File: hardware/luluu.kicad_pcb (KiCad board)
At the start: 4 copper layers, 75 x 30 mm, 55 parts, among them J1 BATT_CON, J2 RPi SWD, J3 STEMMA_{QT} I_{2}C, J4 Micro_SD_Card, J6 USB_C_Receptacle_USB2.0, J7 DISP_LCD_ST7789, Q1 AO3401A, Q2 BSS138, SW1 SW_USBBOOT, SW2 SW_RESET, SW3 SW_POWER, U1 W25Q128JVSS, U2 RT9080-33GJ5, U3 RP2040, U4 TP4054-42, Y1 X322512MSB4SI

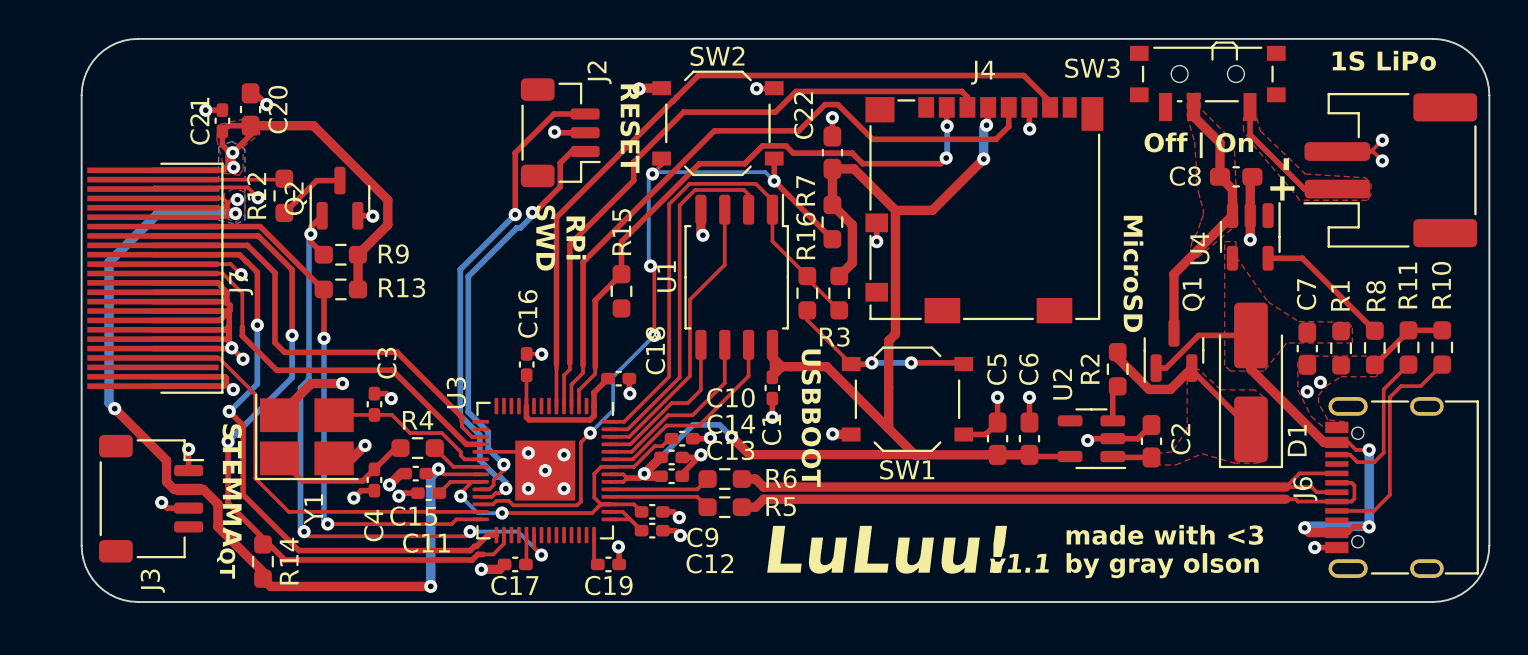
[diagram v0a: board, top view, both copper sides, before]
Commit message: pcb rev 2.0 progress
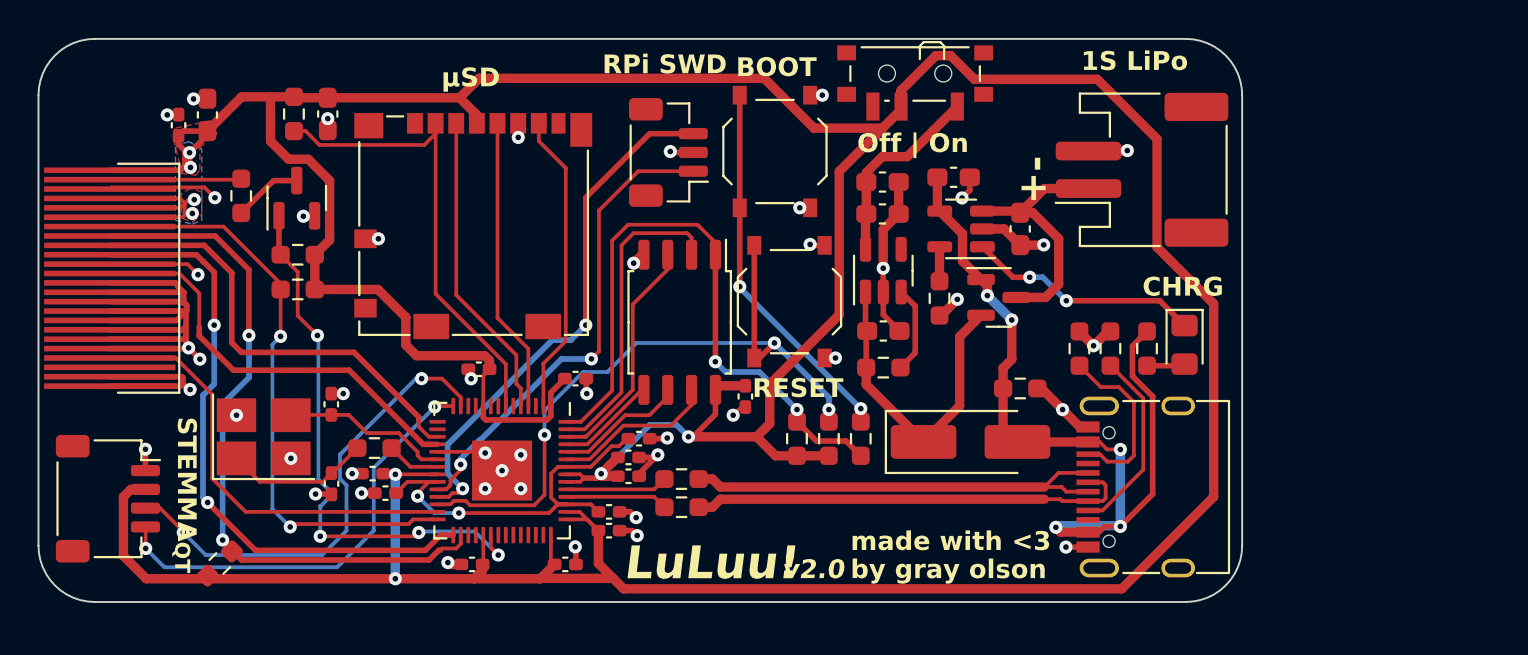
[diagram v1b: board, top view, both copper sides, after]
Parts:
- added D2: CHRG, LED_SMD:LED_0805_2012Metric_Pad1.15x1.40mm_HandSolder, F.Cu at (171.0, 94.5)
- added R17: 1k, Resistor_SMD:R_0603_1608Metric_Pad0.98x0.95mm_HandSolder, F.Cu at (169.0, 94.8)
- moved J4 27.3 mm to (133.1, 88.2)
- moved C22 27.0 mm to (125.3, 82.2), turned to -90 degrees
- moved R8 23.3 mm to (157.9, 92.1)
- moved C7 20.9 mm to (158.7, 85.6), turned to 0 degrees
- moved R15 19.8 mm to (123.5, 82.2), turned to 90 degrees
- moved R10 17.7 mm to (167.1, 94.8)
- moved R11 17.5 mm to (165.4, 94.8)
- moved R1 17.2 mm to (162.2, 96.9), turned to 180 degrees
- moved SW3 15.6 mm to (156.6, 80.4)
- moved C2 15.4 mm to (154.9, 93.8), turned to 0 degrees
- moved U4 15.4 mm to (159.1, 88.4), turned to 180 degrees
- moved D1 15.3 mm to (159.6, 99.7), turned to 0 degrees
- moved C5 15.0 mm to (154.9, 85.9), turned to 0 degrees
- moved SW1 15.0 mm to (149.2, 84.2), turned to 90 degrees
- moved C6 14.3 mm to (154.9, 87.6), turned to 0 degrees
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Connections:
- C5 pad 1: +3V3 -> Net-(SW3-A)
- C6 pad 1: +3V3 -> Net-(SW3-A)
- J1 pad 1: Net-(J1-Pin_1) -> +BATT
- SW3 pad 1: Net-(J1-Pin_1) -> Net-(SW3-A)
- SW3 pad 2: +BATT -> +3V3
- U2 pad 5: +3V3 -> Net-(SW3-A)
- U3 pad 2: unconnected-(U3-GPIO0-Pad2) -> /CARD_SPI_{MISO}
- U3 pad 3: /CARD_~{CS} -> unconnected-(U3-GPIO1-Pad3)
- U3 pad 6: /CARD_SPI_{MISO} -> unconnected-(U3-GPIO4-Pad6)
- U3 pad 7: unconnected-(U3-GPIO5-Pad7) -> /CARD_~{CS}
- U4 pad 1: unconnected-(U4-~{CHRG}-Pad1) -> Net-(D2-K)
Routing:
- net +3V3: track 176.8 -> 266.1 mm, vias 11 -> 8
- net /CARD_SPI_{MISO}: track 40.7 -> 16.2 mm
- net /I_{2}C_{DATA}: track 1.56 -> 25.5 mm, vias 1 -> 2
- net /I_{2}C_{CLOCK}: track 0.00 -> 23.5 mm, vias 0 -> 2
- net /CARD_SPI_{CLOCK}: track 36.1 -> 15.7 mm
- net +5V: track 26.9 -> 45.0 mm, vias 3 -> 5
- net /CARD_SPI_{MOSI}: track 34.6 -> 16.5 mm
- net Net-(D2-K): track 0.00 -> 12.5 mm, vias 0 -> 2
- net GND: track 117.5 -> 106.0 mm
- net /USB_D+: track 35.0 -> 23.7 mm
- net /USB_D-: track 34.6 -> 23.7 mm
- net Net-(SW3-A): track 0.00 -> 10.4 mm
- net Net-(R16-Pad1): track 9.88 -> 20.1 mm
- net Net-(J1-Pin_1): track 7.32 -> 0.00 mm
- net /CARD_~{CS}: track 32.4 -> 25.3 mm, vias 2 -> 0
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- removed copper zone on F.Cu, net +5V
- removed copper zone on F.Cu, net +BATT
- removed copper zone on F.Cu, net GND
- removed copper zone on F.Cu, net Net-(D1-K)
- removed copper zone on F.Cu, net Net-(J1-Pin_1)
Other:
- board size 75 x 30 mm -> 64.1 x 30 mm
- board text added: "BOOT"
- board text added: "CHRG"
- board text added: "v2.0"
- board text added: "µSD"
- board text removed: "MicroSD"
- board text removed: "USBBOOT"
- board text removed: "v1.1"
